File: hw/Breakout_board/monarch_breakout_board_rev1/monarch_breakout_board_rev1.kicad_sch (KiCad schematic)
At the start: 26 parts, among them U2 FDC2214RGHR, U3 INA226AQDGSRQ1, U4 INA226AQDGSRQ1

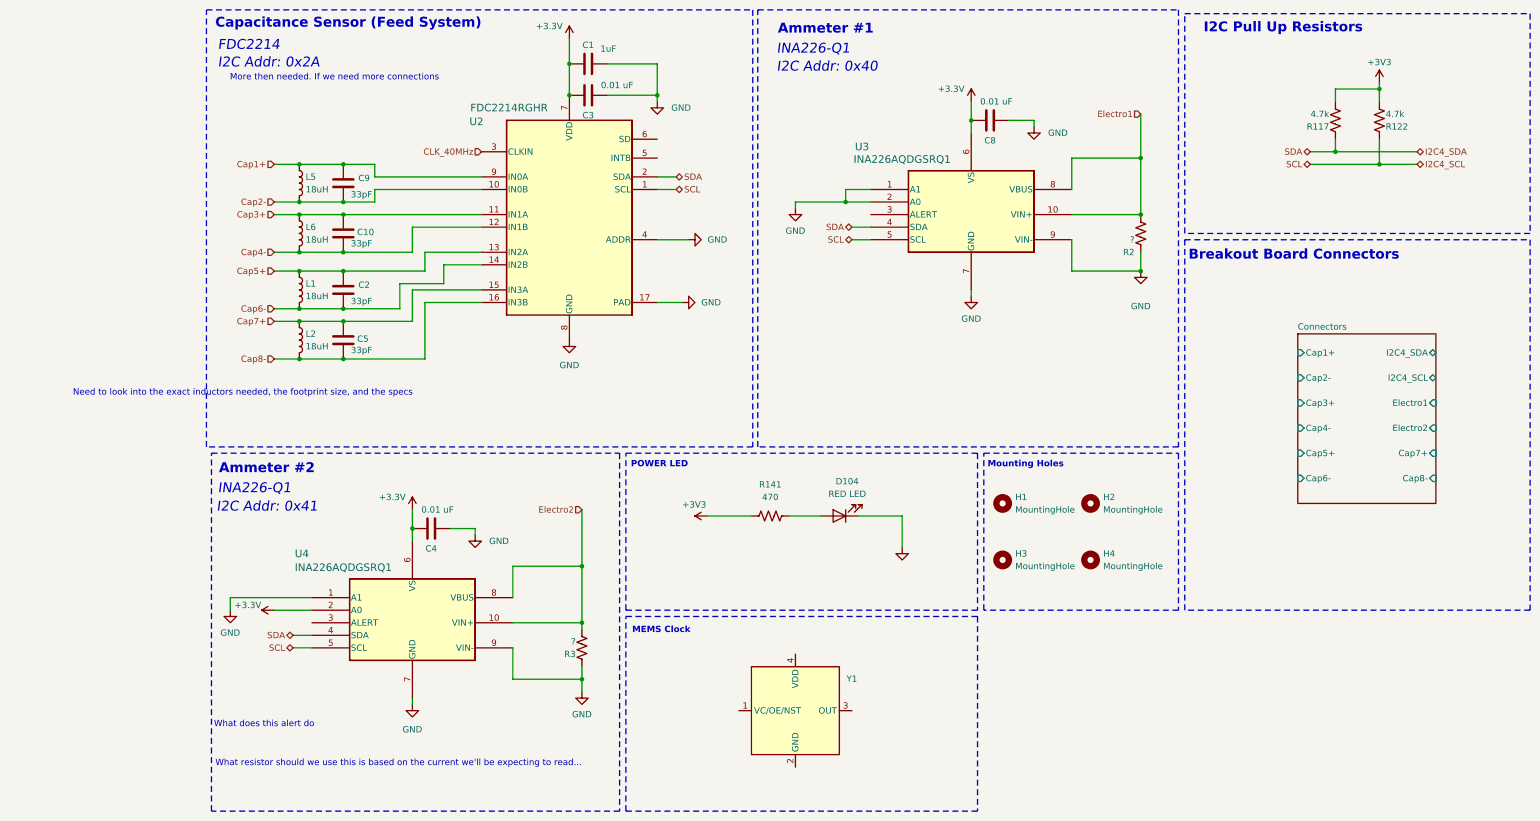
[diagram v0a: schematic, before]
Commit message: Breakout Board History Fix
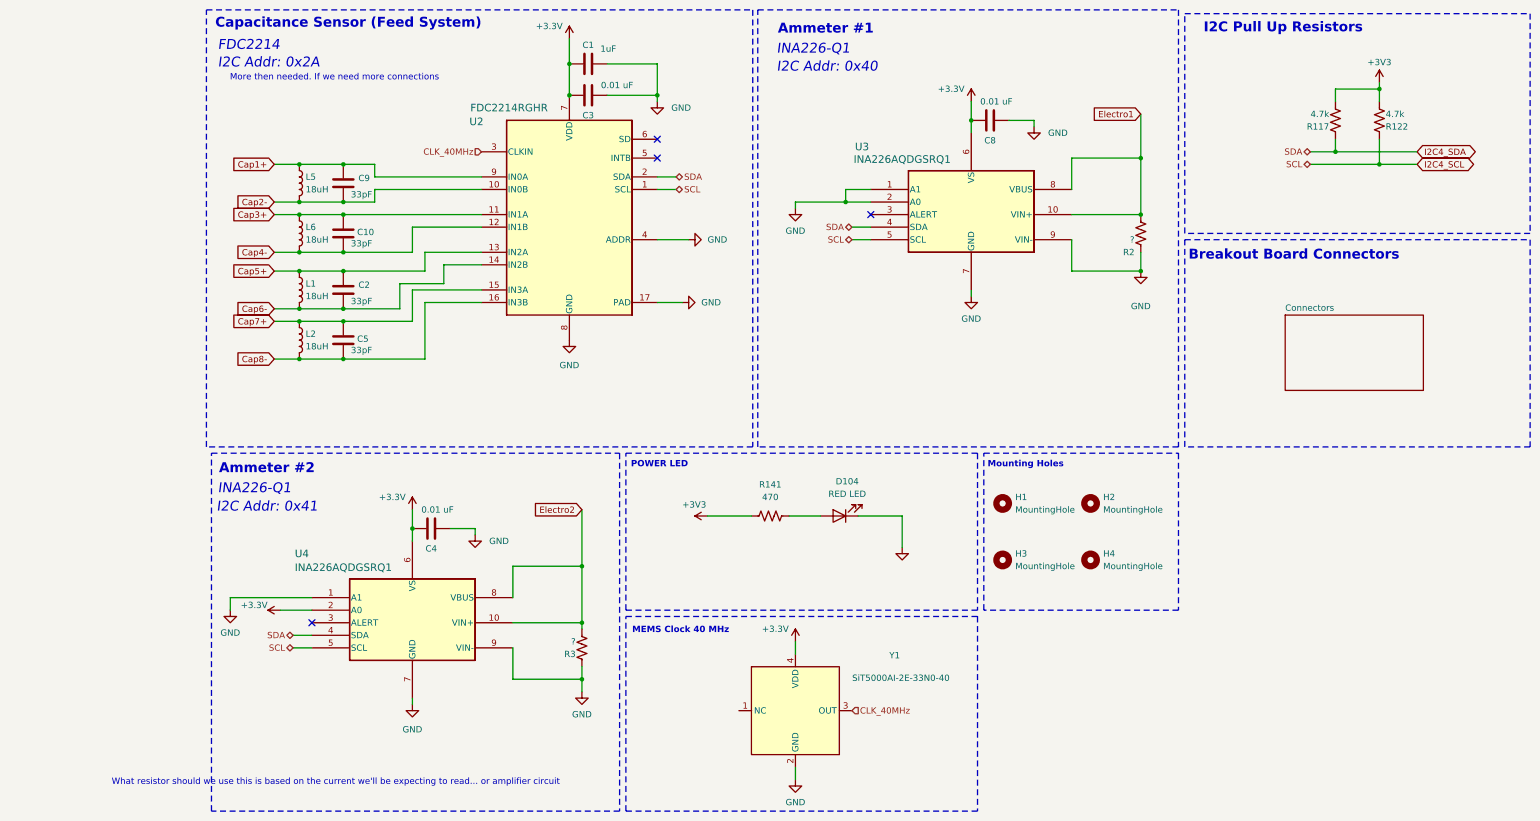
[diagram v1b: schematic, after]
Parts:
- H1, H2, H3, H4: footprint (none) -> MountingHole:MountingHole_2.2mm_M2_DIN965_Pad
- Y1: value ~ -> SiT5000AI-2E-33N0-40; footprint (none) -> Oscillator:Oscillator_SMD_SiT_PQFN-4Pin_3.2x2.5mm
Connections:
- net +3.3V: now also Y1.4 (VDD)
- net CLK_40MHz: now also Y1.3 (OUT)
- net GND: now also Y1.2 (GND)
- no-connect marks 0 -> 4
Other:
- sheet Connectors ports: added none; removed Cap1+, Cap2-, Cap3+, Cap4-, Cap5+, Cap6-, Cap7+, Cap8-, Electro1, Electro2, I2C4_SCL, I2C4_SDA
- note added: "MEMS Clock 40 MHz"
- note added: "What resistor should we use this is based on the current we'll be expecting to read... or amplifier circuit"
- note removed: "MEMS Clock"
- note removed: "Need to look into the exact inductors needed, the footprint size, and the specs"
- note removed: "What does this alert do"
- note removed: "What resistor should we use this is based on the current we'll be expecting to read..."

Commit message: Revert "Crystal Clock Completion, All Pins Assigned, More Routing Work"
This reverts commit 432819c756e1f3cf9abb2627b488983cb7a3cfe3
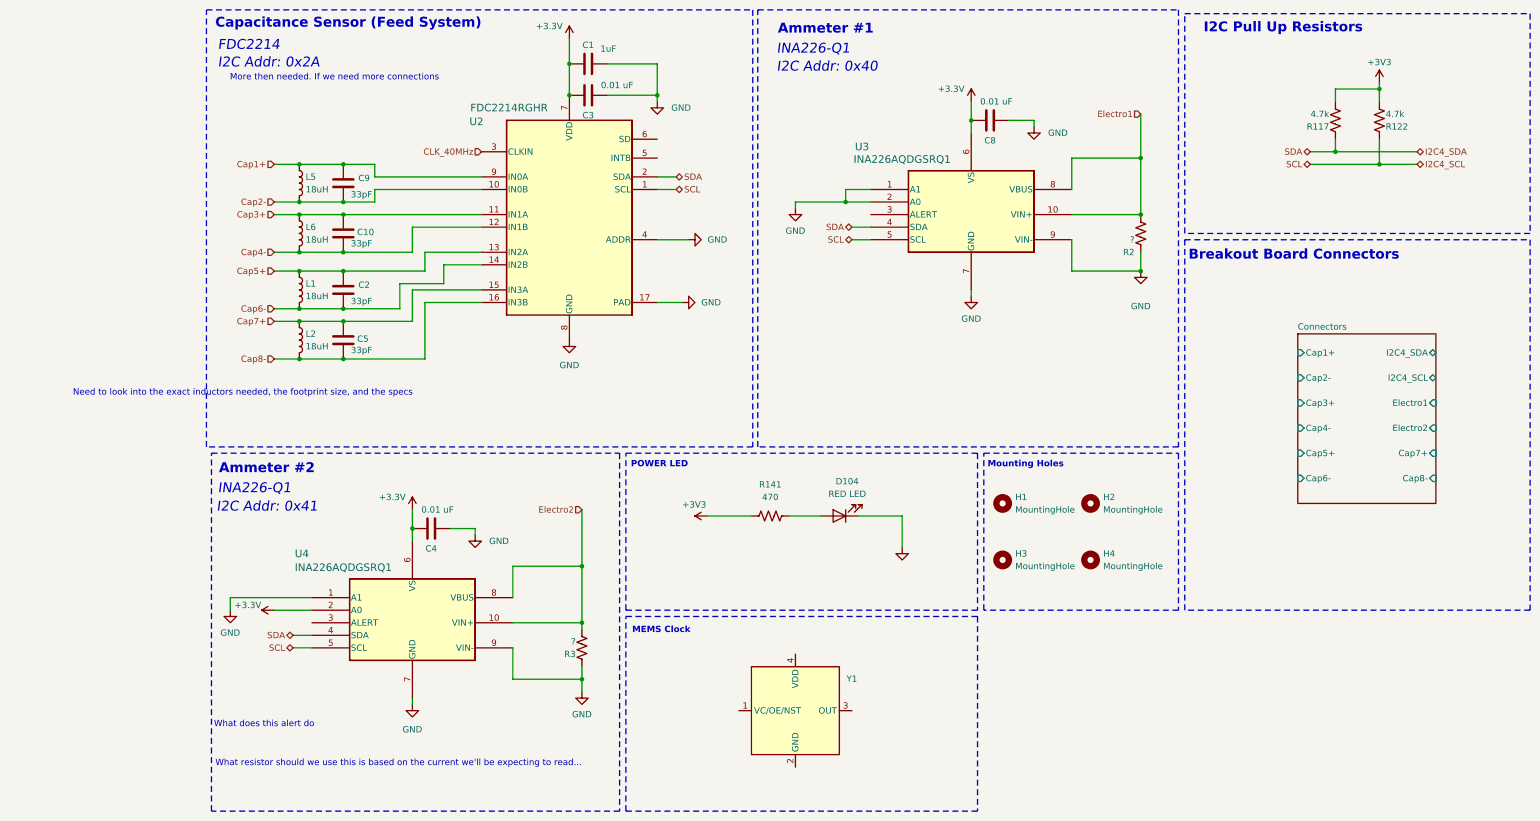
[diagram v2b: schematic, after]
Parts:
- H1, H2, H3, H4: footprint MountingHole:MountingHole_2.2mm_M2_DIN965_Pad -> (none)
- Y1: value SiT5000AI-2E-33N0-40 -> ~; footprint Oscillator:Oscillator_SMD_SiT_PQFN-4Pin_3.2x2.5mm -> (none)
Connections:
- net +3.3V: no longer Y1.4 (VDD)
- net CLK_40MHz: no longer Y1.3 (OUT)
- net GND: no longer Y1.2 (GND)
- no-connect marks 4 -> 0
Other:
- sheet Connectors ports: added Cap1+, Cap2-, Cap3+, Cap4-, Cap5+, Cap6-, Cap7+, Cap8-, Electro1, Electro2, I2C4_SCL, I2C4_SDA; removed none
- note added: "MEMS Clock"
- note added: "Need to look into the exact inductors needed, the footprint size, and the specs"
- note added: "What does this alert do"
- note added: "What resistor should we use this is based on the current we'll be expecting to read..."
- note removed: "MEMS Clock 40 MHz"
- note removed: "What resistor should we use this is based on the current we'll be expecting to read... or amplifier circuit"
